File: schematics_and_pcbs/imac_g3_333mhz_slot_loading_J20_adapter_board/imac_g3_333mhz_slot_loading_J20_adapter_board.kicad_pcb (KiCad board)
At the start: 2 copper layers, 82.6 x 51.7 mm, 12 parts, among them J1 DB15_Female_HighDensity, J20 Conn_02x10_Odd_Even, U1 ATmega328-PU, U2 ATmega328-PU, Y1 Crystal, Y2 Crystal

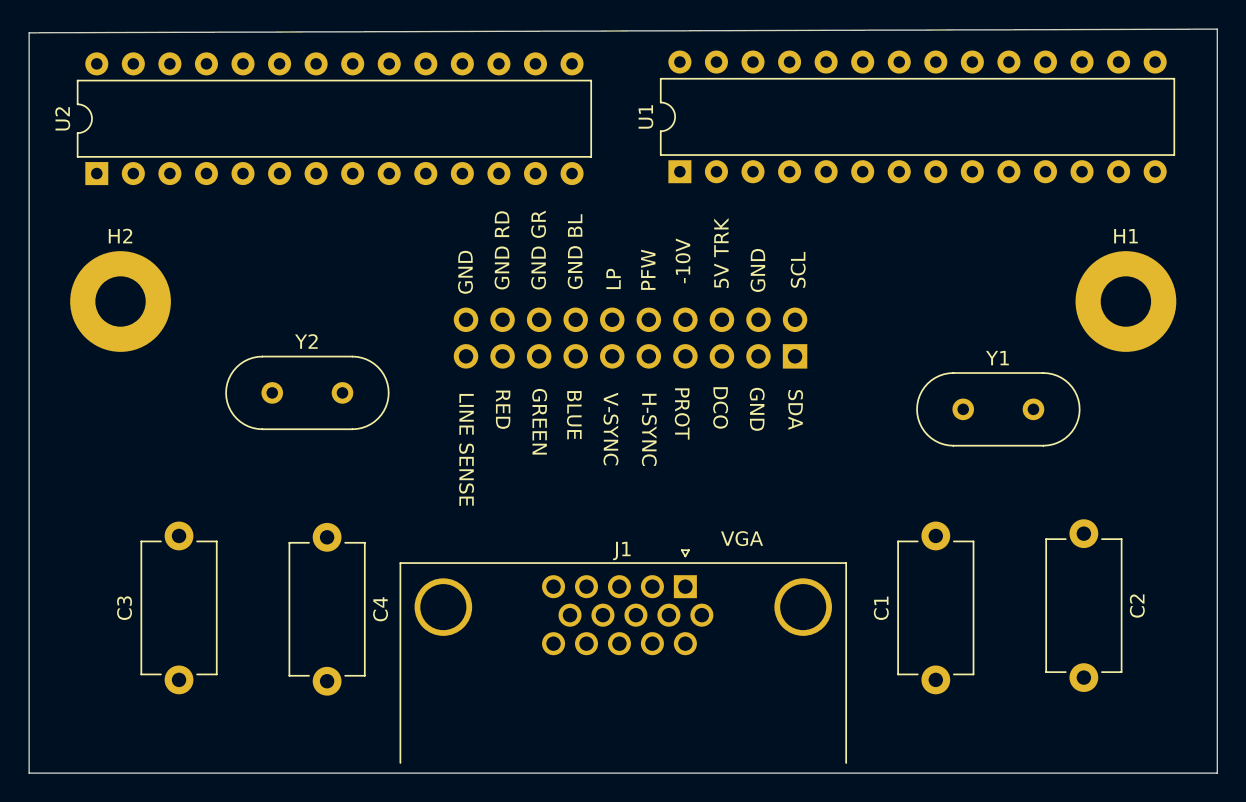
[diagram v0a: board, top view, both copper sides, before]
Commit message: made board a little curvier
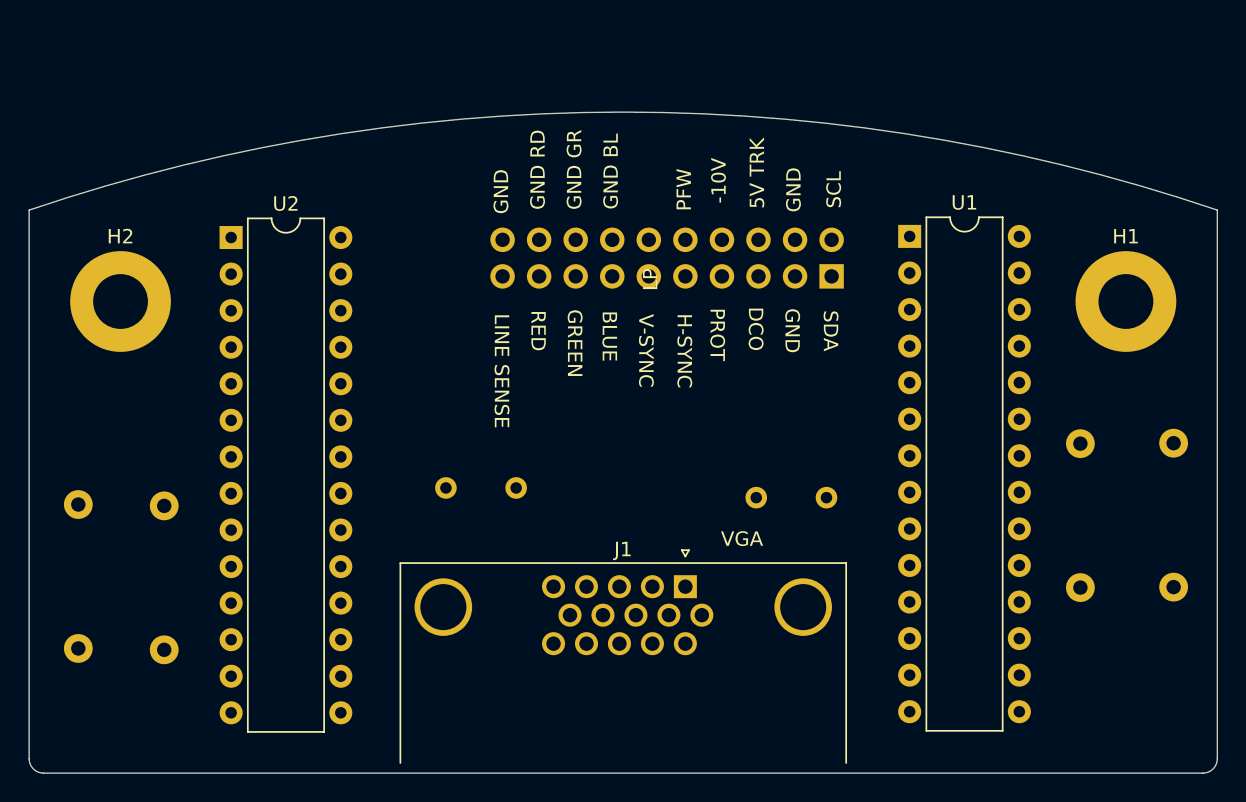
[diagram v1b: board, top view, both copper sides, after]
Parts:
- C1, C2, C3, C4, Y1, Y2: moved to B.Cu
- moved U1 16.6 mm to (194.5, 65.3), turned to 0 degrees
- moved Y2 13.8 mm to (162.3, 82.8)
- moved C1 11.9 mm to (206.4, 89.7)
- moved C4 11.5 mm to (142.7, 84.0)
- moved Y1 11.3 mm to (188.7, 83.5), turned to 180 degrees
- moved U2 10.3 mm to (147.4, 65.4), turned to 0 degrees
- moved C2 8.85 mm to (212.9, 79.7)
- moved C3 7.33 mm to (136.8, 94.0)
- moved J20 6.11 mm to (189.1, 68.1)
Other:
- board size 82.6 x 51.7 mm -> 82.6 x 45.9 mm
